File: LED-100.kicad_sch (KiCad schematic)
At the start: 99 parts, among them J2 LDA100_2_J2, J3 LDA100_2_J3, J4 LDA100_2_J4, J5 xtra, J7 Conn_01x01, J8 Conn_01x06, SW1 SW_SPDT, U1 TLC5947DAP, U2 TLC5947DAP, U3 TLC5947DAP, U4 TEENSY 4.0

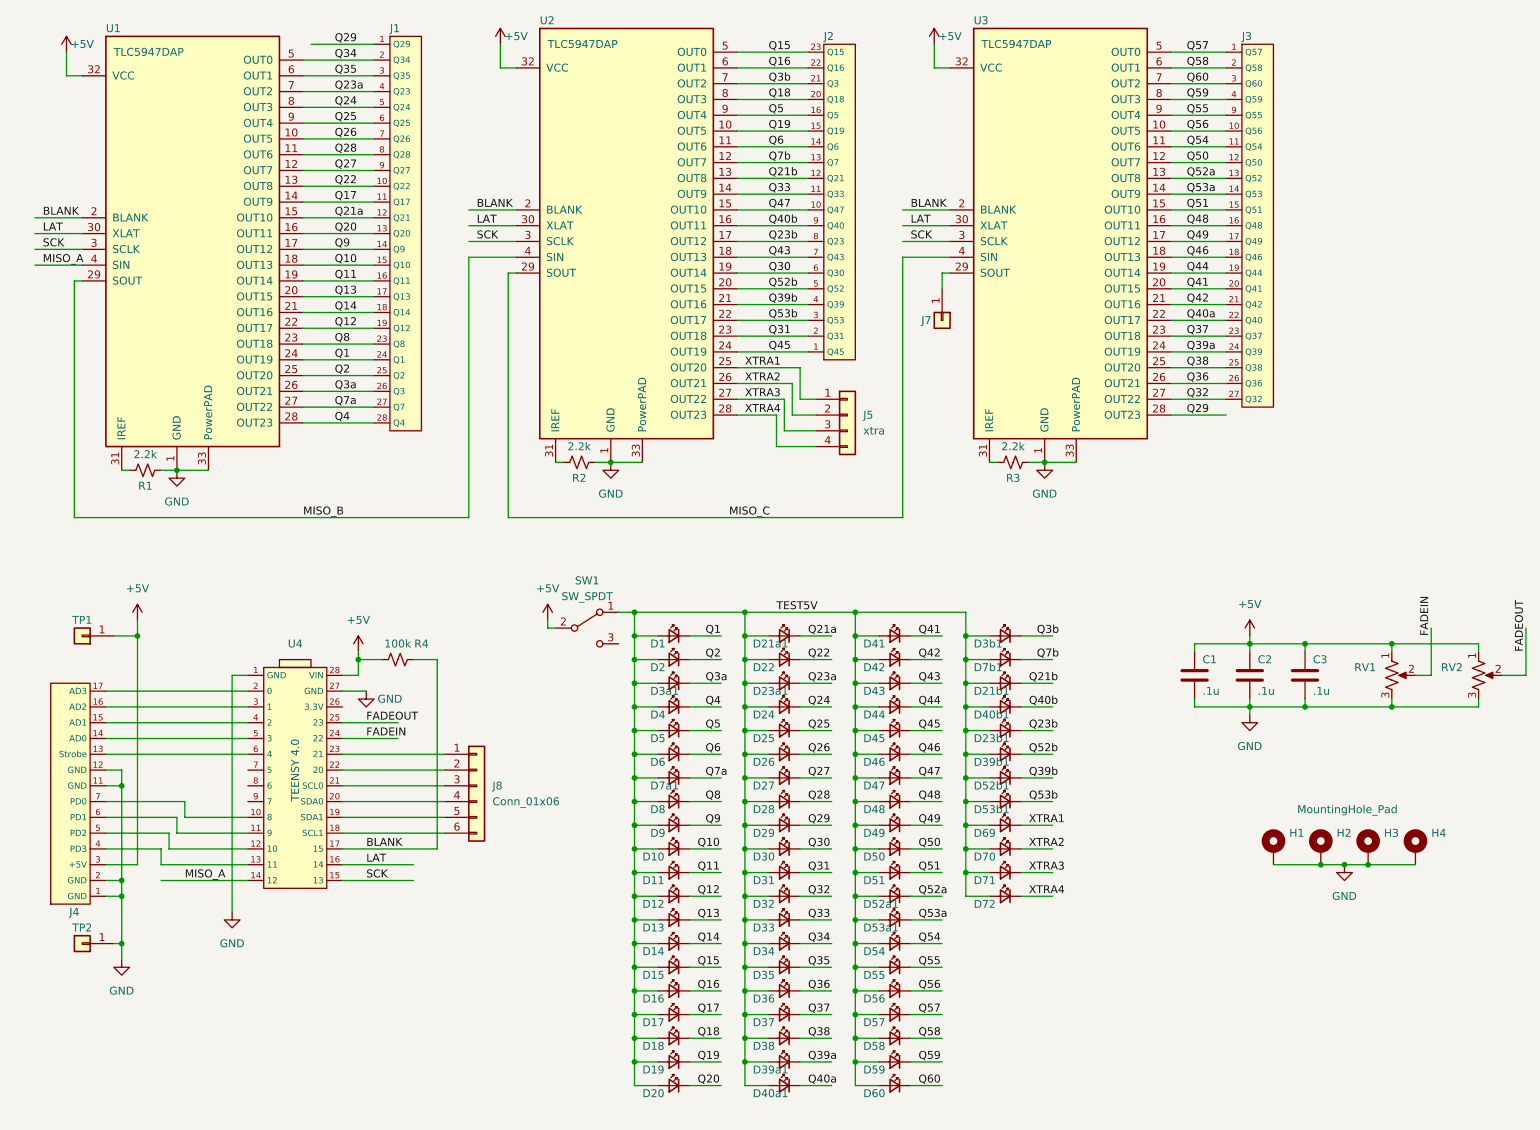
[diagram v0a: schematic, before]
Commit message: tweaks & cleanup
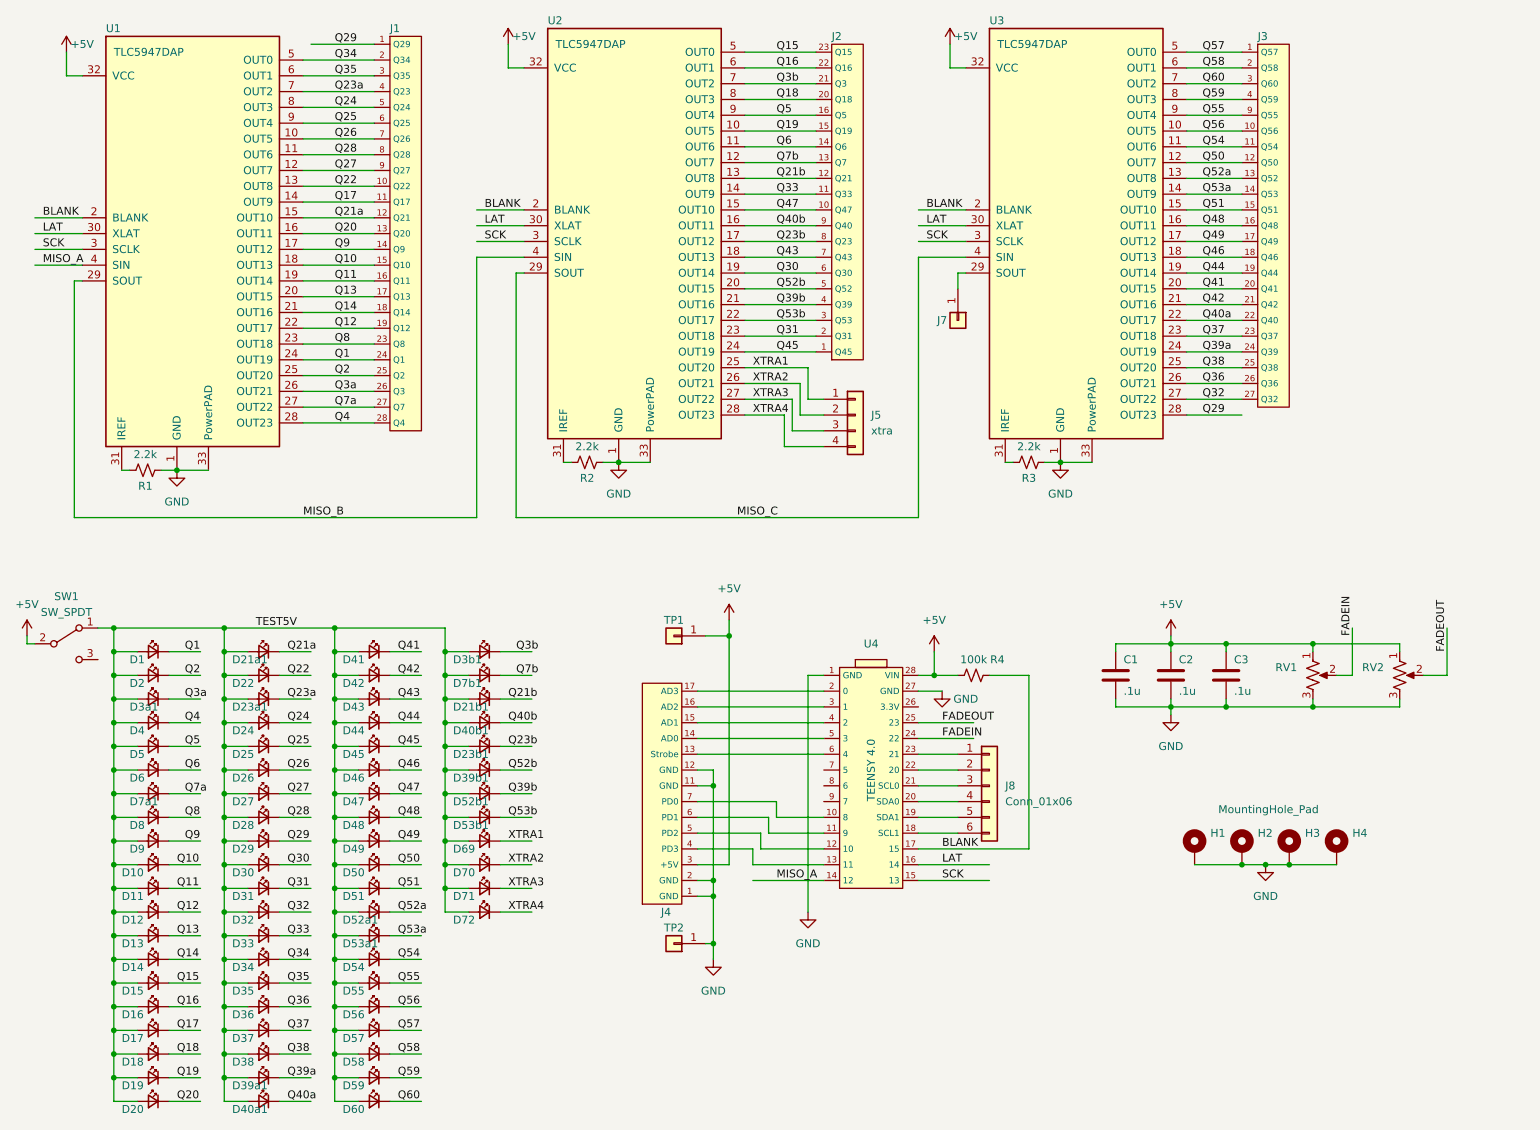
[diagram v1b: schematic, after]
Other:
- company: (none) -> Duhan Power!
- title: (none) -> LED-100
- moved on the sheet: C1, C2, C3, D1, D10, D11, D12, D13, D14, D15, D16, D17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
